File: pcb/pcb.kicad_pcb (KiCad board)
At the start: 4 copper layers, 57.5 x 21.5 mm, 13 parts, among them J1 Conn_Coaxial, U1 XIAO-nRF52840-SMD, U2 NEO-M9V-20B, U3 AP2112K-3.3

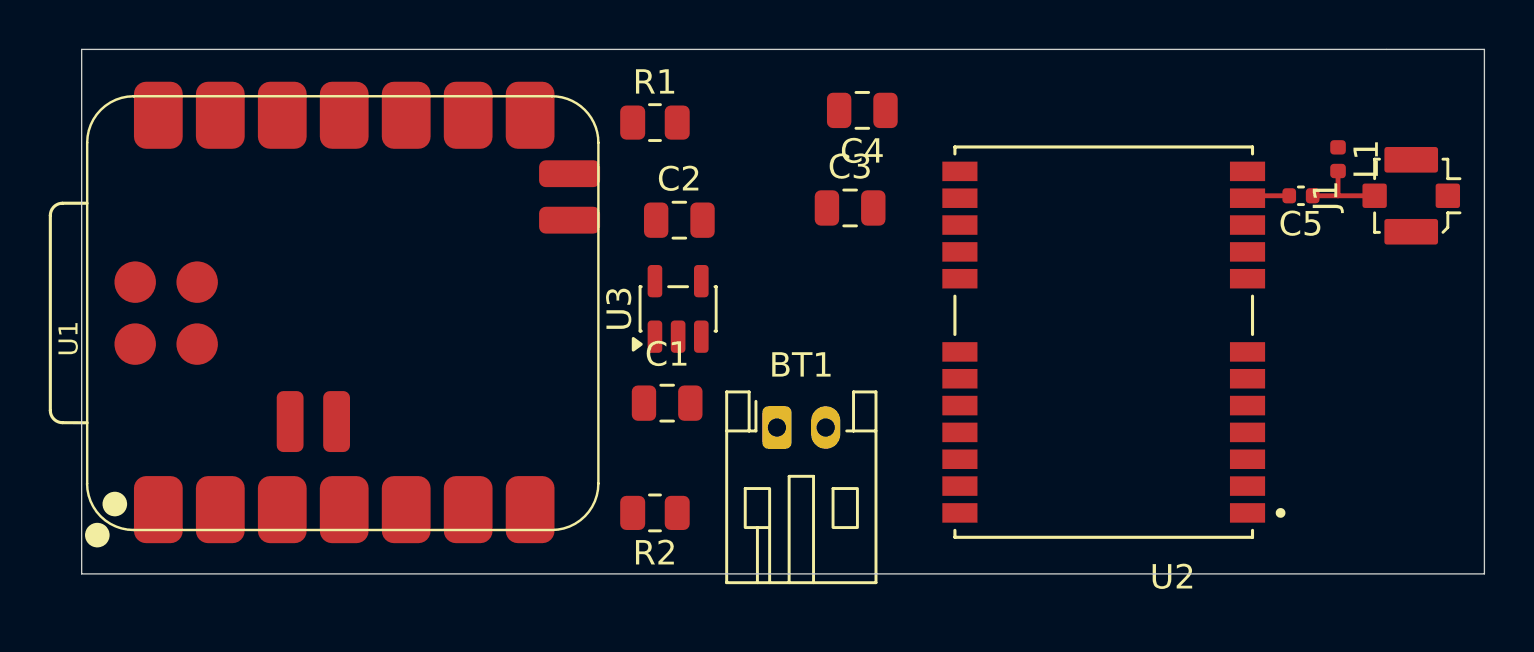
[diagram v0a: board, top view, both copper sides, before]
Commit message: first version pcb done
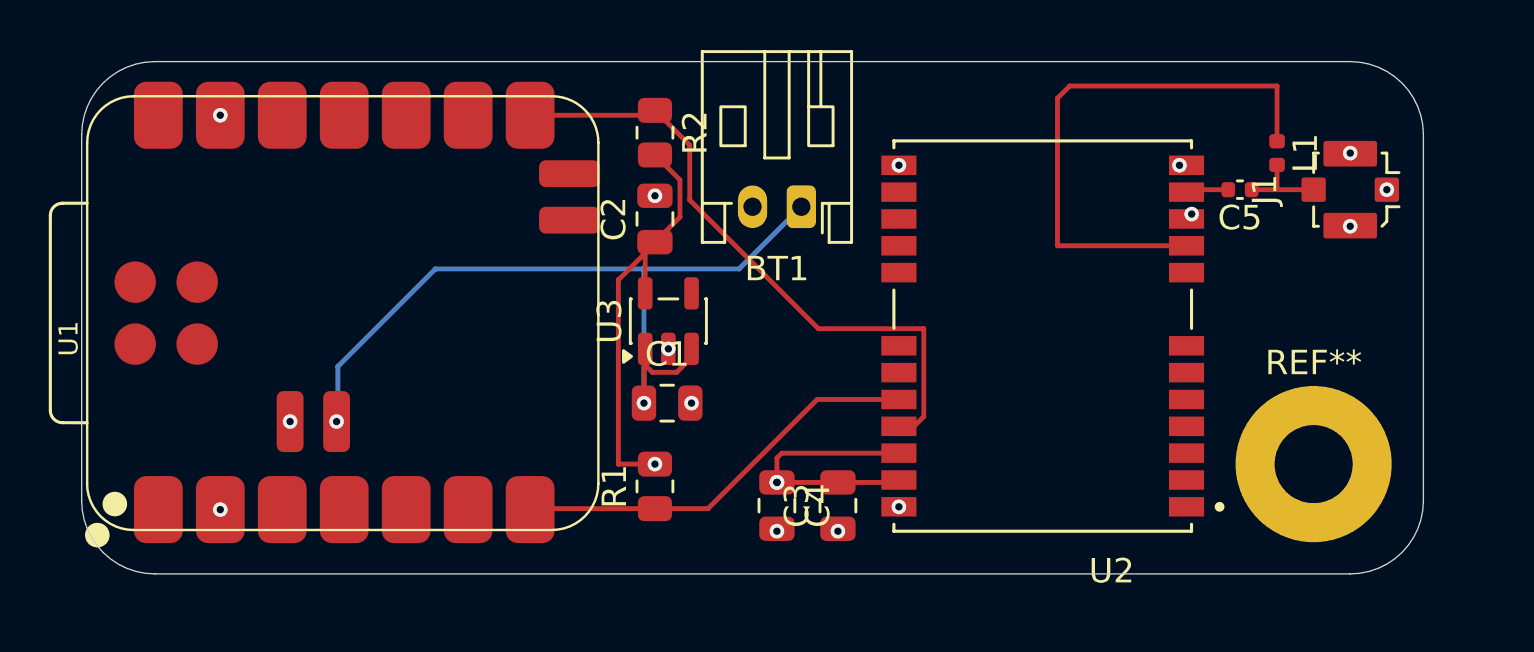
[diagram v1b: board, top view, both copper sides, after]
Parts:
- added REF**: MountingHole_3.2mm_M3_Pad, MountingHole:MountingHole_3.2mm_M3_Pad, F.Cu at (108.0, 66.5)
- moved C4 16.6 mm to (86.0, 68.2), turned to -90 degrees
- moved R2 15.6 mm to (81.0, 52.9), turned to -90 degrees
- moved R1 14.9 mm to (81.0, 67.4), turned to 90 degrees
- moved C3 12.2 mm to (88.5, 68.2), turned to 90 degrees
- moved BT1 9.11 mm to (87.0, 56.0), turned to 180 degrees
- moved C5 2.51 mm to (105.0, 55.2)
- moved J1 2.51 mm to (109.5, 55.2)
- moved L1 2.51 mm to (106.5, 53.8)
- moved U2 2.51 mm to (96.9, 61.2)
- moved C2 1.00 mm to (81.0, 56.5), turned to 90 degrees
- moved U3 0.64 mm to (81.5, 60.6)
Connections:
- L1 pad 1: Net-(U2-VCC) -> Net-(U2-VCC_RF)
- R1 pad 1: Net-(U1-P1.12_D7_RX) -> /uart_tx
- R2 pad 1: Net-(U1-P1.11_D6_TX) -> /uart_rx
- U1 pad 2: unconnected-(U1-P0.03_A1_D1-Pad2) -> GND
- U1 pad 7: Net-(U1-P1.11_D6_TX) -> /uart_tx
- U1 pad 8: Net-(U1-P1.12_D7_RX) -> /uart_rx
- U2 pad 20: Net-(U1-P1.12_D7_RX) -> /uart_tx
- U2 pad 21: Net-(U1-P1.11_D6_TX) -> /uart_rx
- U2 pad 9: unconnected-(U2-VCC_RF-Pad9) -> Net-(U2-VCC_RF)
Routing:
- net GND: track 0.00 -> 105.0 mm, vias 0 -> 15
- net Net-(BT1-+): track 0.00 -> 35.0 mm, vias 0 -> 2
- net Net-(U2-VCC): track 0.00 -> 34.8 mm, vias 0 -> 3
- net /uart_rx: track 0.00 -> 26.3 mm
- net Net-(U2-VCC_RF): track 0.00 -> 22.8 mm
- net /uart_tx: track 0.00 -> 17.0 mm
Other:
- board size 57.5 x 21.5 mm -> 55 x 21 mm
- board text added: "https://github.com/teehee567"
- board text added: "meow"
- board text added: "noob"
